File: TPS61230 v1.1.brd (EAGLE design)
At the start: 25.6 x 11.4 mm, 14 parts

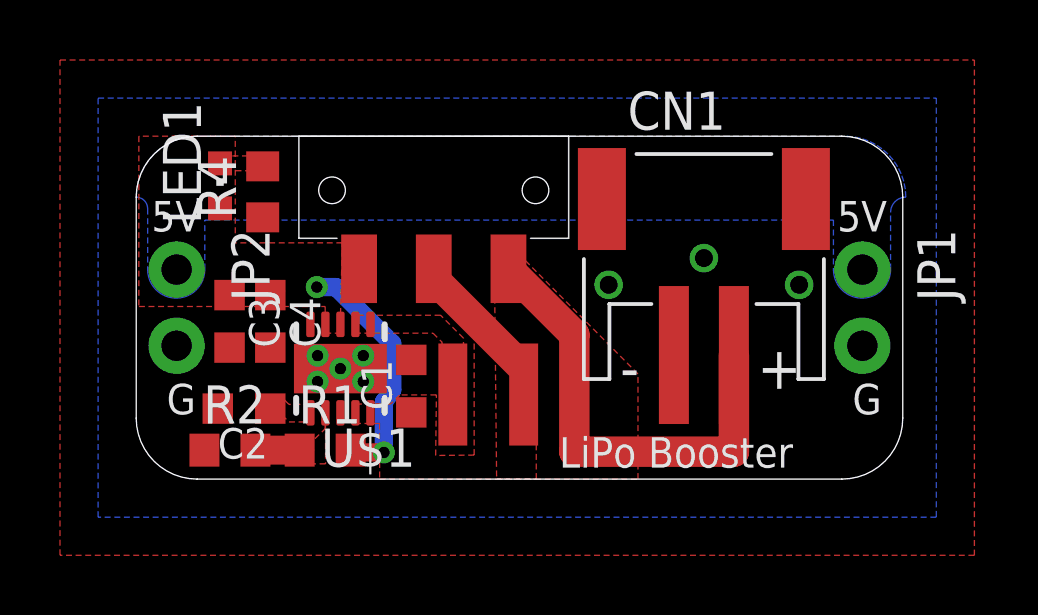
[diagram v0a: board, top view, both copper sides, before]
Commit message: v1.1
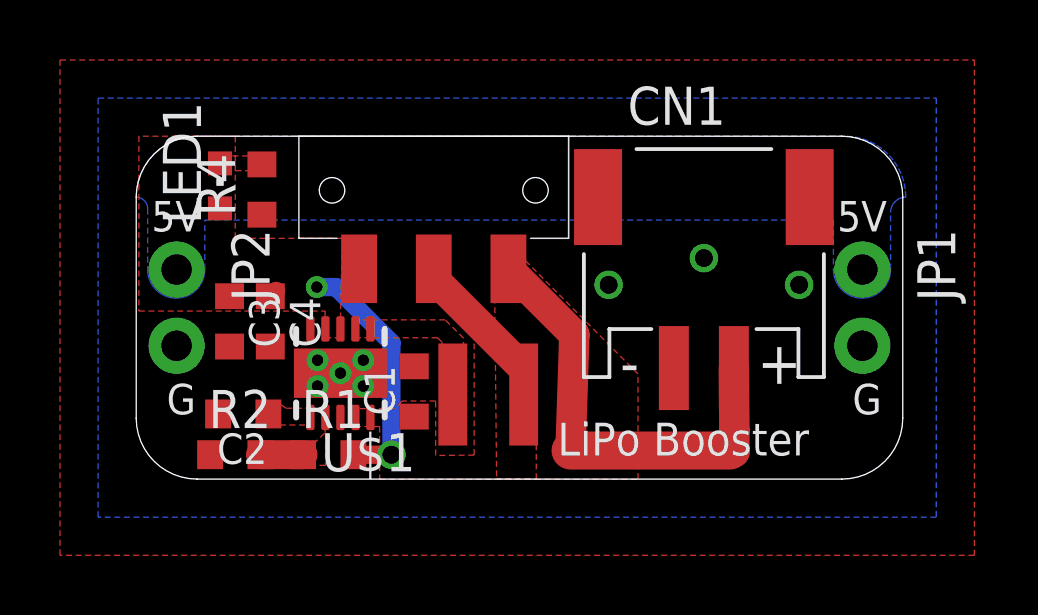
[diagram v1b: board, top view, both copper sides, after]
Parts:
- moved R2 0.23 mm to (3.30, 0.81)
- moved C1 0.20 mm to (9.27, 2.92)
- moved R1 0.18 mm to (6.40, 0.81)
- moved C2 0.18 mm to (3.57, 2.17)
- moved CN1 0.17 mm to (18.9, 8.00)
- moved U$1 0.15 mm to (6.81, 3.53)
- moved R4 0.08 mm to (4.19, 9.65)
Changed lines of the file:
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@@
 <setting verticaltext="up"/>
 </settings>
-<grid distance="0.05" unitdist="inch" unit="mm" style="lines" multiple="1" display="yes" altdistance="0.005" altunitdist="inch" altunit="inch"/>
+<grid distance="0.005" unitdist="inch" unit="inch" style="lines" multiple="1" display="yes" altdistance="0.001" altunitdist="inch" altunit="inch"/>
 <layers>
 <layer number="1" name="Top" color="4" fill="1" visible="yes" active="yes"/>
@@
 <wire x1="0" y1="9.398" x2="2.032" y2="11.43" width="0.0254" layer="20" curve="-90"/>
 <wire x1="2.032" y1="0" x2="0" y2="2.032" width="0.0254" layer="20" curve="-90"/>
-<text x="14.097" y="0.381" size="1.016" layer="21">LiPo Booster</text>
+<text x="14.0462" y="0.7874" size="1.0922" layer="21">LiPo Booster</text>
 <text x="23.368" y="8.255" size="1.016" layer="21">5V</text>
 <text x="0.508" y="8.255" size="1.016" layer="21">5V</text>
@@
 <param name="mdViaViaSameLayer" value="8mil"/>
 <param name="mnLayersViaInSmd" value="2"/>
-<param name="mdCopperDimension" value="15mil"/>
+<param name="mdCopperDimension" value="12mil"/>
 <param name="mdDrill" value="6mil"/>
 <param name="mdSmdStop" value="0mil"/>
@@
 <param name="mvStopFrame" value="1"/>
 <param name="mvCreamFrame" value="0"/>
-<param name="mlMinStopFrame" value="3mil"/>
-<param name="mlMaxStopFrame" value="3mil"/>
+<param name="mlMinStopFrame" value="0mil"/>
+<param name="mlMaxStopFrame" value="0mil"/>
 <param name="mlMinCreamFrame" value="0mil"/>
 <param name="mlMaxCreamFrame" value="0mil"/>
@@
 </autorouter>
 <elements>
-<element name="U$1" library="texas" package="DRC-S-PVSON-N11" value="TPS61230" x="6.8072" y="3.683" rot="R180"/>
+<element name="U$1" library="texas" package="DRC-S-PVSON-N11" value="TPS61230" x="6.8072" y="3.5306" rot="R180"/>
 <element name="L1" library="Coilcraft" package="XFL4020" value="1uH" x="11.7348" y="2.8194" rot="R180"/>
-<element name="C1" library="adafruit" package="C0603K" value="22uF" x="9.1694" y="3.0988" rot="R90"/>
-<element name="C2" library="adafruit" package="C0603K" value="10nF" x="3.5941" y="2.3495" rot="R180"/>
-<element name="R1" library="adafruit" package="R0603" value="402k" x="6.2992" y="0.9652"/>
-<element name="R2" library="adafruit" package="R0603" value="100k" x="3.1242" y="0.9652"/>
+<element name="C1" library="adafruit" package="C0603K" value="22uF" x="9.271" y="2.921" rot="R90"/>
+<element name="C2" library="adafruit" package="C0603K" value="10nF" x="3.5687" y="2.1717" rot="R180"/>
+<element name="R1" library="adafruit" package="R0603" value="402k" x="6.4008" y="0.8128"/>
+<element name="R2" library="adafruit" package="R0603" value="100k" x="3.302" y="0.8128"/>
 <element name="C3" library="adafruit" package="C0603K" value="22uF" x="3.1115" y="5.2578" rot="R270"/>
 <element name="C4" library="adafruit" package="C0603K" value="22uF" x="4.4704" y="5.2578" rot="R270"/>
-<element name="CN1" library="adafruit" package="JST-PH-2-SMT-RA" value="" x="18.923" y="7.8359"/>
+<element name="CN1" library="adafruit" package="JST-PH-2-SMT-RA" value="" x="18.923" y="8.001"/>
 <element name="JP1" library="SparkFun-Connectors" package="1X02_NO_SILK" value="M021X02_NO_SILK" x="24.2062" y="6.985" locked="yes" rot="R270"/>
 <element name="JP2" library="SparkFun-Connectors" package="1X02_NO_SILK" value="M021X02_NO_SILK" x="1.3462" y="6.985" locked="yes" rot="R270"/>
 <element name="U$2" library="C&amp;K Components" package="JS102011" value="SWITCH-SPDT" x="9.9187" y="8.1534" rot="R180"/>
 <element name="LED1" library="adafruit" package="CHIPLED_0603" value="" x="2.794" y="9.77391875"/>
-<element name="R4" library="adafruit" package="R0603" value="1k" x="4.2164" y="9.5758" rot="R90"/>
+<element name="R4" library="adafruit" package="R0603" value="1k" x="4.191" y="9.652" rot="R90"/>
 </elements>
 <signals>
@@
 <contactref element="L1" pad="P$2"/>
 <polygon width="0.254" layer="1" thermals="no">
-<vertex x="7.2898" y="5.461"/>
-<vertex x="7.2898" y="4.8641"/>
-<vertex x="9.8933" y="4.8641"/>
+<vertex x="7.2898" y="5.3086"/>
+<vertex x="7.2898" y="4.7117"/>
+<vertex x="10.0457" y="4.7117"/>
 <vertex x="10.1981" y="4.5593"/>
 <vertex x="10.1981" y="4.3688"/>
 <vertex x="10.9093" y="4.3688"/>
 <vertex x="10.9093" y="4.699"/>
-<vertex x="10.1473" y="5.461"/>
+<vertex x="10.2997" y="5.3086"/>
 </polygon>
 </signal>
@@
 <wire x1="12.8778" y1="2.8575" x2="12.9159" y2="2.8194" width="0.8128" layer="1"/>
 <polygon width="0.254" layer="1" thermals="no" rank="3">
-<vertex x="7.2898" y="2.5019"/>
-<vertex x="7.2898" y="1.8542"/>
-<vertex x="8.1153" y="1.8542"/>
+<vertex x="7.2898" y="2.3495"/>
+<vertex x="7.2898" y="1.7526"/>
+<vertex x="8.1153" y="1.7526"/>
 <vertex x="8.1153" y="0"/>
 <vertex x="13.335" y="0"/>
@@
 <vertex x="11.2649" y="0.8001"/>
 <vertex x="9.9822" y="0.7874"/>
-<vertex x="10.0076" y="2.8067"/>
-<vertex x="8.7884" y="2.8067"/>
-<vertex x="8.4836" y="2.5019"/>
+<vertex x="9.9822" y="2.6035"/>
+<vertex x="8.8646" y="2.6035"/>
+<vertex x="8.6106" y="2.3495"/>
 </polygon>
 </signal>
@@
 <contactref element="C2" pad="1"/>
 <polygon width="0.254" layer="1" thermals="no">
-<vertex x="5.7912" y="2.4892"/>
-<vertex x="5.0927" y="2.4892"/>
-<vertex x="4.8641" y="2.7178"/>
-<vertex x="4.8641" y="2.1336"/>
-<vertex x="5.0927" y="1.905"/>
-<vertex x="5.7912" y="1.905"/>
+<vertex x="5.842" y="2.3622"/>
+<vertex x="4.9911" y="2.3622"/>
+<vertex x="4.7879" y="2.5146"/>
+<vertex x="4.7879" y="1.8034"/>
+<vertex x="5.842" y="1.8034"/>
 </polygon>
 </signal>
@@
 </polygon>
 <polygon width="0.254" layer="1" thermals="no" rank="2">
-<vertex x="6.7945" y="4.8641"/>
-<vertex x="6.8707" y="7.874"/>
-<vertex x="3.302" y="7.874"/>
+<vertex x="6.7945" y="4.7117"/>
+<vertex x="6.8707" y="8.0264"/>
+<vertex x="3.302" y="8.0264"/>
 <vertex x="3.302" y="11.43"/>
 <vertex x="0.0889" y="11.43"/>
-<vertex x="0.0889" y="5.7531"/>
-<vertex x="6.2992" y="5.7531"/>
-<vertex x="6.2992" y="4.8641"/>
-</polygon>
-<wire x1="7.1492" y1="0.9652" x2="7.2254" y2="0.889" width="0.6096" layer="1"/>
-<wire x1="7.2254" y1="0.889" x2="8.255" y2="0.889" width="0.6096" layer="1"/>
-<via x="8.255" y="0.889" extent="1-16" drill="0.381"/>
-<wire x1="8.255" y1="0.889" x2="8.255" y2="2.5654" width="0.6096" layer="16"/>
-<wire x1="8.255" y1="2.5654" x2="8.5344" y2="2.9718" width="0.6096" layer="16"/>
-<wire x1="8.5344" y1="2.9718" x2="8.5344" y2="4.5212" width="0.6096" layer="16"/>
-<wire x1="8.5344" y1="4.5212" x2="6.6548" y2="6.4008" width="0.6096" layer="16"/>
+<vertex x="0.0889" y="5.6007"/>
+<vertex x="6.2992" y="5.6007"/>
+<vertex x="6.2992" y="4.7117"/>
+</polygon>
+<wire x1="7.239" y1="0.8128" x2="7.2254" y2="0.889" width="0.6096" layer="1"/>
 <wire x1="6.6548" y1="6.4008" x2="6.0198" y2="6.4008" width="0.6096" layer="16"/>
 <via x="6.0198" y="6.4008" extent="1-16" drill="0.381"/>
-<wire x1="4.6622" y1="6.2738" x2="4.4704" y2="6.1328" width="0.6096" layer="1"/>
+<wire x1="4.6622" y1="6.2738" x2="4.4704" y2="6.096" width="0.6096" layer="1"/>
+<wire x1="6.6548" y1="6.4008" x2="8.509" y2="4.5466" width="0.6096" layer="16"/>
+<wire x1="8.509" y1="4.5466" x2="8.509" y2="0.8128" width="0.6096" layer="16"/>
+<via x="8.509" y="0.8128" extent="1-16" drill="0.6"/>
+<wire x1="8.509" y1="0.8128" x2="7.239" y2="0.8128" width="0.6096" layer="1"/>
 </signal>
 <signal name="N$6">
@@
 <contactref element="R1" pad="1"/>
 <contactref element="U$1" pad="7"/>
-<wire x1="3.9742" y1="0.9652" x2="5.4492" y2="0.9652" width="0.9652" layer="1"/>
+<wire x1="4.1402" y1="0.8128" x2="5.5626" y2="0.8128" width="0.9652" layer="1"/>
 <polygon width="0.254" layer="1" thermals="no">
-<vertex x="5.3975" y="1.3462"/>
-<vertex x="5.9563" y="1.3462"/>
-<vertex x="6.2992" y="1.6764"/>
+<vertex x="5.08" y="1.1684"/>
+<vertex x="5.9055" y="1.1684"/>
+<vertex x="6.2992" y="1.5494"/>
 <vertex x="6.2992" y="1.8415"/>
 <vertex x="6.3119" y="1.8415"/>
-<vertex x="6.3119" y="0.508"/>
-<vertex x="5.1054" y="0.508"/>
-<vertex x="5.08" y="1.2446"/>
+<vertex x="6.3119" y="0.4572"/>
+<vertex x="5.08" y="0.4572"/>
 </polygon>
 </signal>
@@
 <contactref element="CN1" pad="1" route="any" routetag="G$1.2"/>
 <contactref element="U$2" pad="P$3"/>
-<wire x1="19.923" y1="4.1359" x2="19.923" y2="0.9144" width="1.016" layer="1"/>
-<wire x1="19.923" y1="0.9144" x2="14.605" y2="0.9144" width="1.016" layer="1"/>
-<wire x1="14.605" y1="0.9144" x2="14.605" y2="4.8133" width="1.016" layer="1"/>
+<wire x1="19.923" y1="3.701" x2="19.939" y2="1.6256" width="1.016" layer="1"/>
+<wire x1="19.939" y1="1.6256" x2="19.939" y2="0.9017" width="1.016" layer="1"/>
+<wire x1="19.939" y1="0.9017" x2="19.796" y2="0.9525" width="1.016" layer="1"/>
+<wire x1="19.796" y1="0.9525" x2="14.478" y2="0.9525" width="1.27" layer="1"/>
+<wire x1="14.478" y1="0.9525" x2="14.605" y2="4.8133" width="1.016" layer="1"/>
 <wire x1="14.605" y1="4.8133" x2="12.4079" y2="7.0104" width="1.016" layer="1"/>
 <polygon width="0.254" layer="1" thermals="no" rank="4">
